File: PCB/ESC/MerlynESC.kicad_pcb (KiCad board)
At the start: 6 copper layers, 30.5 x 31.9 mm, 155 parts, among them M1 BLDC Motor, M2 BLDC Motor, M3 BLDC Motor, M4 BLDC Motor, Q1 JMSL0302AU, Q10 JMSL0302AU, Q11 JMSL0302AU, Q12 JMSL0302AU, Q13 JMSL0302AU, Q14 JMSL0302AU, Q15 JMSL0302AU, Q16 JMSL0302AU, Q17 JMSL0302AU, Q18 JMSL0302AU, Q19 JMSL0302AU, Q2 JMSL0302AU, Q20 JMSL0302AU, Q21 JMSL0302AU, Q22 JMSL0302AU, Q23 JMSL0302AU, Q24 JMSL0302AU, Q3 JMSL0302AU, Q4 JMSL0302AU, Q5 JMSL0302AU, Q6 JMSL0302AU, Q7 JMSL0302AU, Q8 JMSL0302AU, Q9 JMSL0302AU, U1 HT75C0-1, U10 EG6288, U11 EFM8BB21F16G, U2 HT7533-1, U3 EFM8BB21F16G, U4 EG6288, U5 EG6288, U6 EFM8BB21F16G, U7 INA139NA, U8 EG6288, U9 EFM8BB21F16G

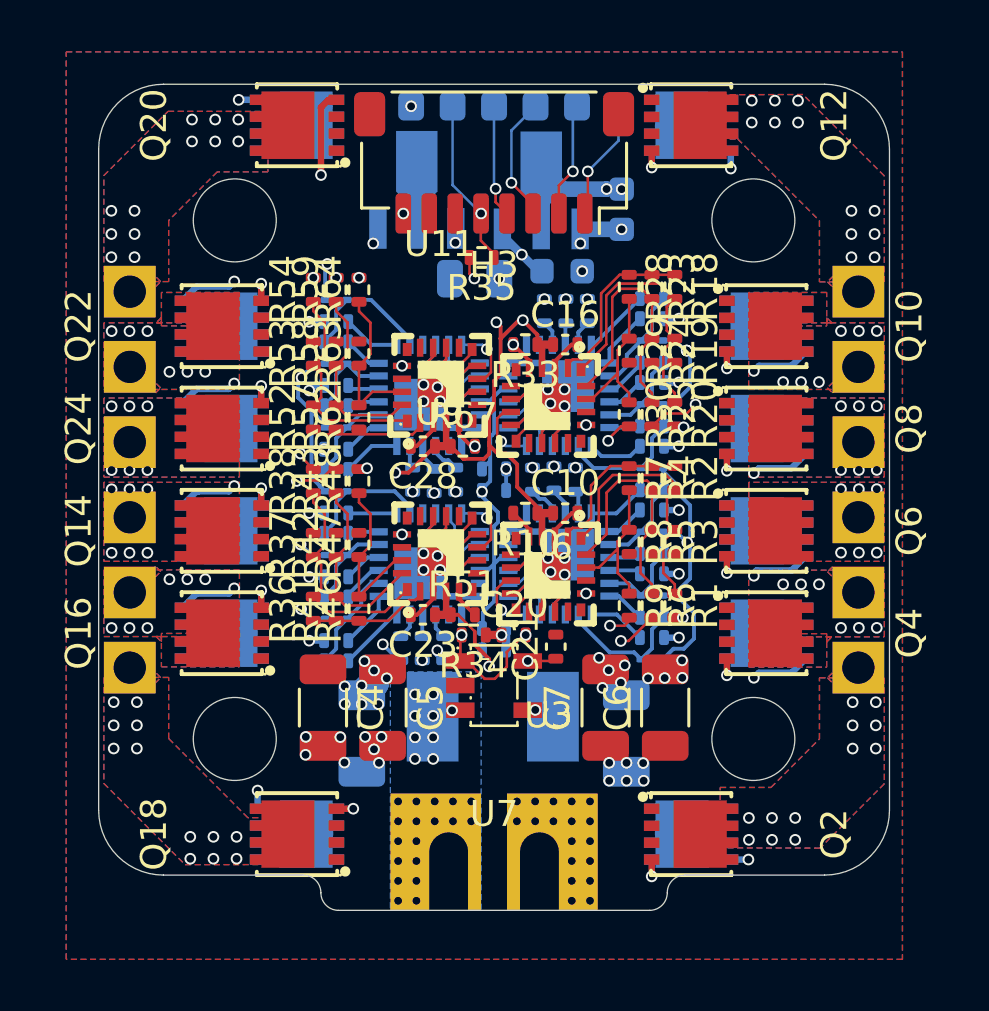
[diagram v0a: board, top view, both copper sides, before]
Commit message: checkpoint
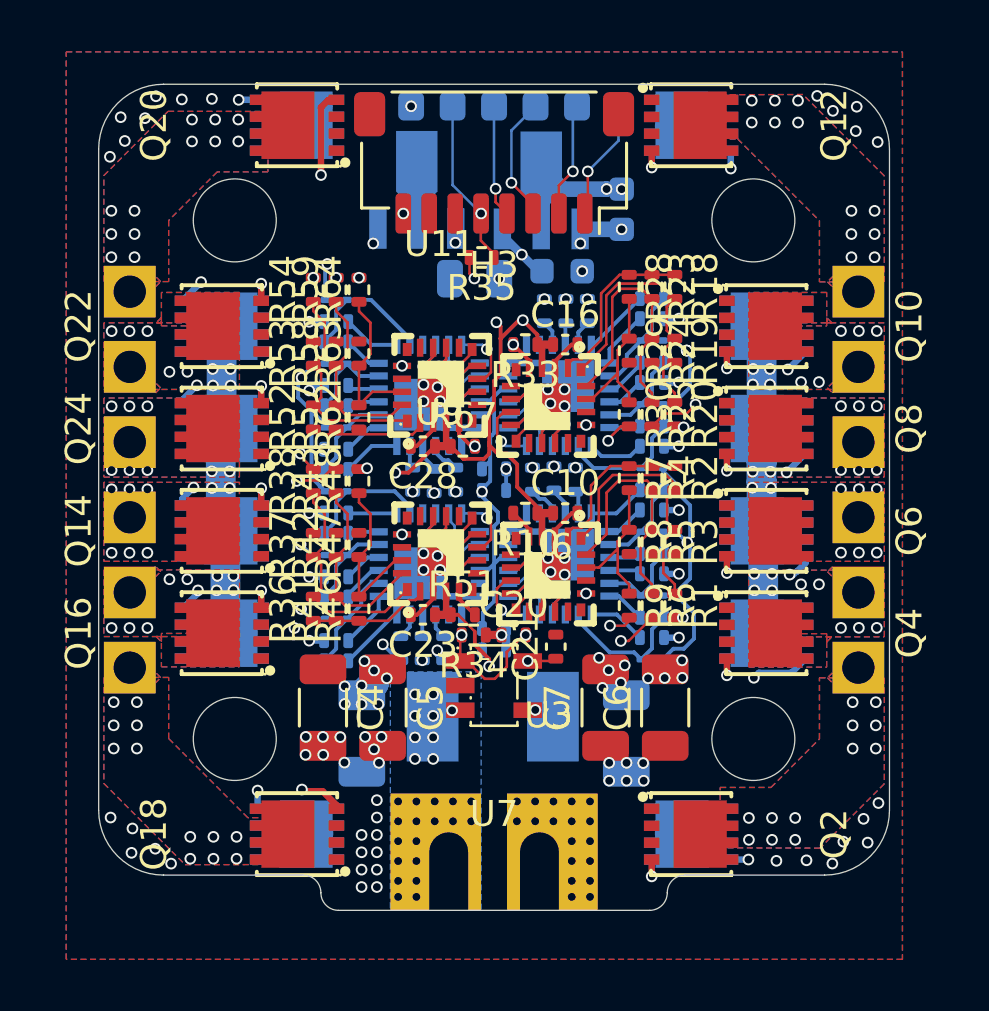
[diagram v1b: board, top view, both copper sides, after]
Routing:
- net +BATT: track 3.82 -> 29.4 mm, vias 19 -> 57
- net Net-(Q18-G): track 9.98 -> 11.7 mm
- net Net-(Q9-G): track 5.95 -> 7.31 mm
- net Net-(Q7-G): track 7.12 -> 8.04 mm
- net Net-(Q15-G): track 5.96 -> 6.80 mm
- net M3_PHASE2: track 8.40 -> 9.22 mm, vias 7 -> 6
- net M1_PHASE2: track 9.08 -> 9.81 mm, vias 7 -> 6
- net M4_PHASE2: track 7.31 -> 8.00 mm, vias 7 -> 6
- net M2_PHASE2: track 5.99 -> 6.47 mm, vias 7 -> 6
- net GND: vias 56 -> 79

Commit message: checkpoint
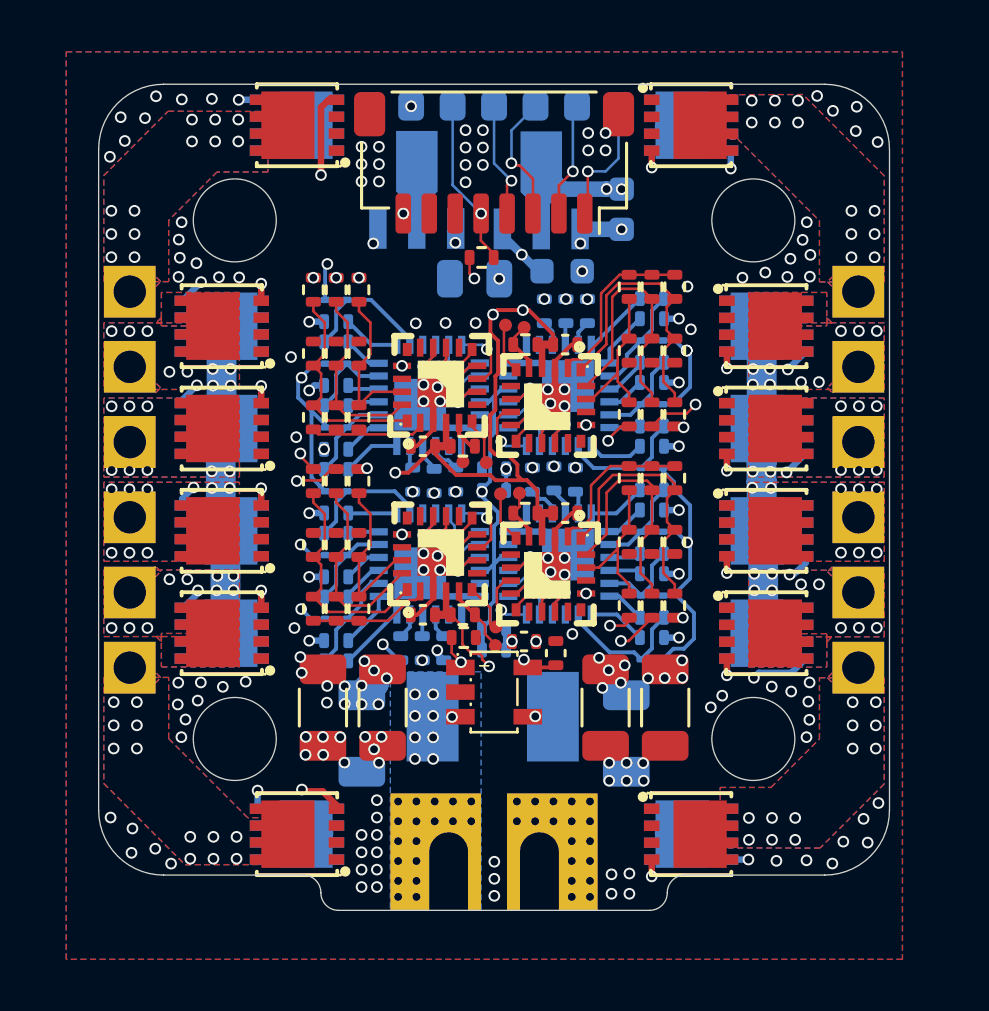
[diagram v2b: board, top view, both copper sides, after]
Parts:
- added H1: C2CK, easyeda2kicad:TestPoint, F.Cu at (156.4, 102.5)
- added H2: C2D, easyeda2kicad:TestPoint, F.Cu at (155.7, 102.5)
- added H4: C2CK, easyeda2kicad:TestPoint, F.Cu at (156.6, 96.1)
- added H5: C2D, easyeda2kicad:TestPoint, F.Cu at (155.9, 96.0)
- added H6: C2CK, easyeda2kicad:TestPoint, F.Cu at (155.5, 108.4)
- added H7: C2D, easyeda2kicad:TestPoint, F.Cu at (155.5, 107.6)
- added H8: C2CK, easyeda2kicad:TestPoint, F.Cu at (154.2, 101.3)
- added H9: C2D, easyeda2kicad:TestPoint, F.Cu at (155.1, 101.3)
- moved C20 0.47 mm to (156.6, 108.2)
- moved R34 0.40 mm to (154.3, 108.0)
- moved C21 0.25 mm to (157.8, 108.6)
- moved U7 0.25 mm to (155.4, 110.1)
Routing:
- net +12V: track 110.8 -> 115.1 mm
- net +3.3V: track 43.1 -> 46.1 mm
- net M1_C2D: track 0.00 -> 1.96 mm
- net M2_C2D: track 0.00 -> 1.94 mm
- net M4_C2D: track 0.00 -> 1.83 mm
- net M3_C2D: track 0.00 -> 1.70 mm
- net M3_C2CK: track 1.15 -> 2.67 mm
- net Net-(U7-OUT): track 20.3 -> 21.7 mm
- net M4_C2CK: track 1.09 -> 2.23 mm, vias 1 -> 0
- net M4_DSHOT: track 18.0 -> 19.1 mm
- net M2_DSHOT: track 15.4 -> 16.5 mm
- net M3_DSHOT: track 23.5 -> 24.6 mm
- net M1_C2CK: track 1.15 -> 2.02 mm
- net M2_C2CK: track 1.15 -> 1.99 mm, vias 1 -> 0
- net GND: track 27.6 -> 28.0 mm, vias 79 -> 123
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
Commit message: checkpoint
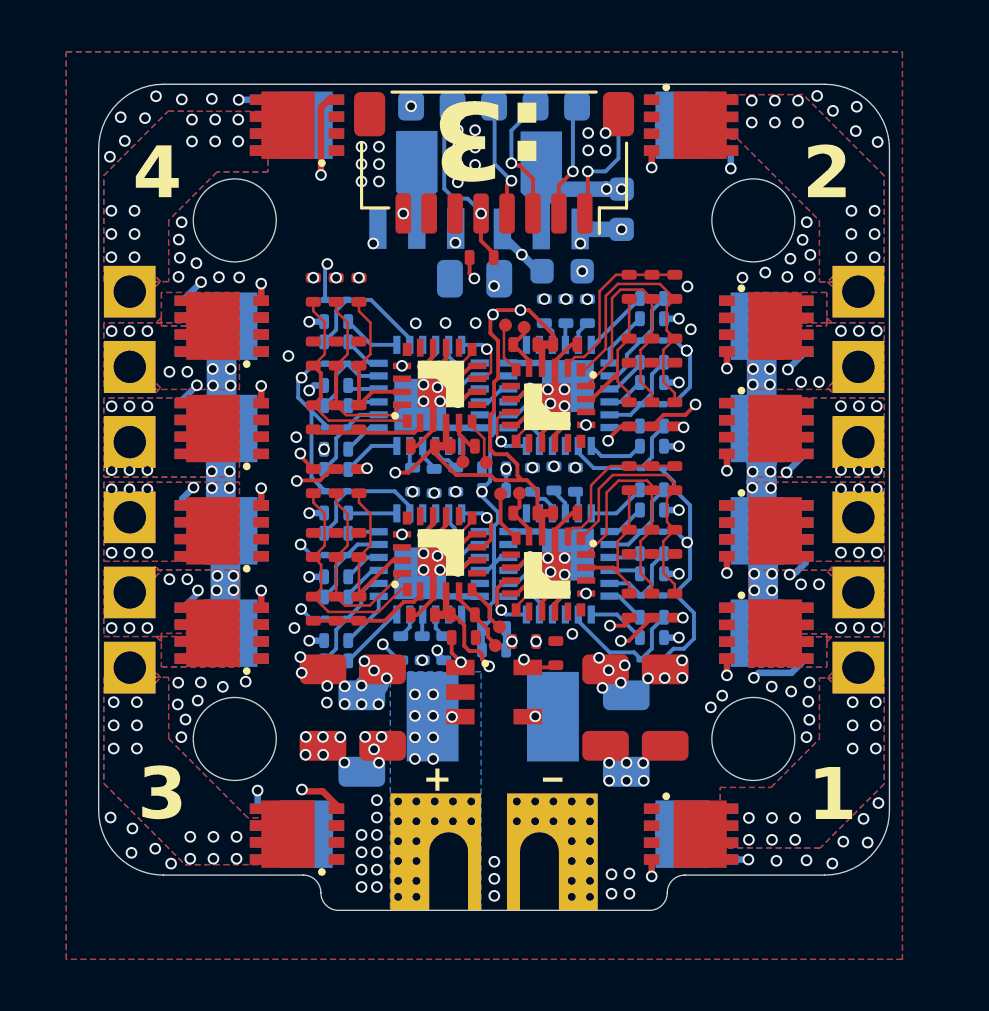
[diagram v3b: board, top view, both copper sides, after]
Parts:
- C1: footprint Capacitor_SMD:C_0805_2012Metric -> easyeda2kicad:C_0805_2012Metric
- C2, C9: footprint Capacitor_SMD:C_0603_1608Metric -> easyeda2kicad:C_0603_1608Metric
- C3, C4, C5, C6, C7, C8: footprint Capacitor_SMD:C_1206_3216Metric -> easyeda2kicad:C_1206_3216Metric
- D1, D10, D11, D12, D2, D3, D4, D5, D6, D7, D8, D9: footprint Diode_SMD:D_SOD-923 -> easyeda2kicad:D_SOD-923
- moved H7 0.14 mm to (155.6, 107.6)
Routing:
- net +BATT: track 29.4 -> 30.2 mm
- net M3_PHASE1: track 10.3 -> 9.65 mm
- net CSense: track 6.49 -> 7.06 mm
- net M3_PHASE2: track 9.22 -> 8.71 mm
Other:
- board text added: "+"
- board text added: "-"
- board text added: "1"
- board text added: "2"
- board text added: "3"
- board text added: "4"
- board text added: ":3"
- board text added: "MerlynESC"
